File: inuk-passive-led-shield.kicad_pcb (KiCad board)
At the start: 2 copper layers, 100 x 27 mm, 13 parts, among them J1 Conn_01x04_Male, J2 Conn_01x10_Male, J3 Conn_01x02_Male, U1 Logo_NM

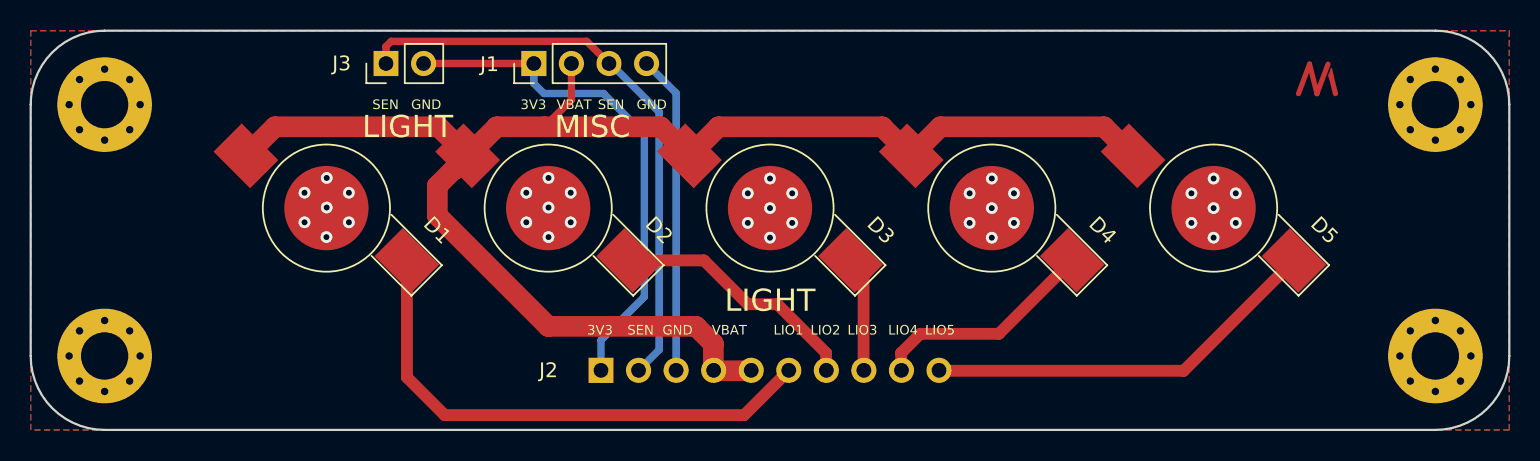
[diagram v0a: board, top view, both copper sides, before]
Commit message: created production files
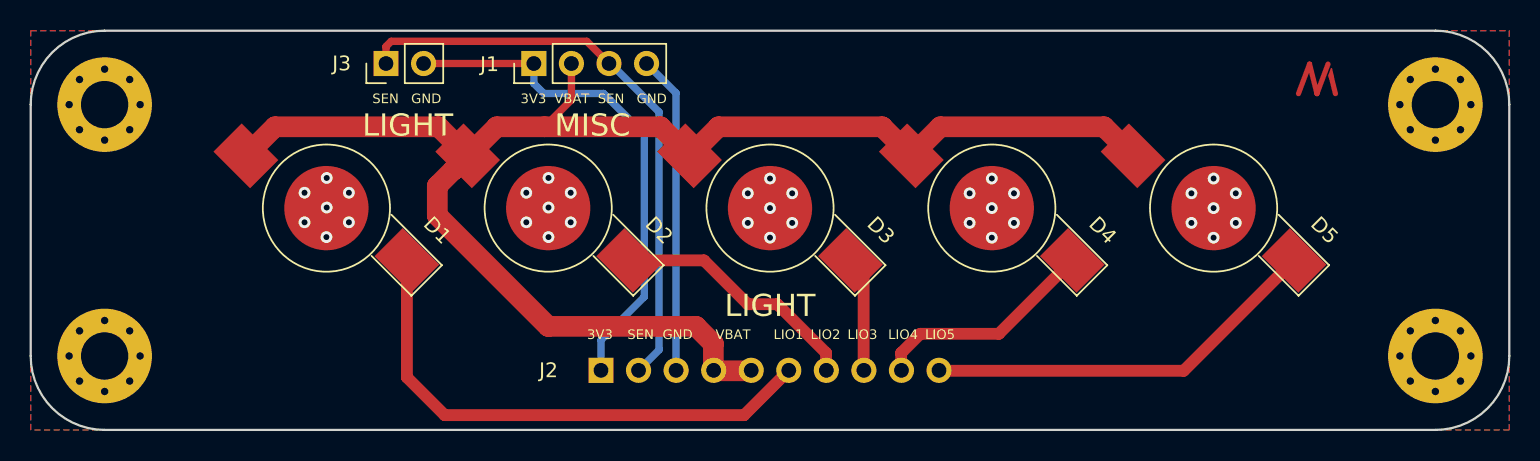
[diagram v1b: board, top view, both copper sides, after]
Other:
- board text added: "Rev: 1.0"
- board text removed: "Rev: 0.9"
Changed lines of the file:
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@@
     (visible_elements FFFFFF7F)
     (pcbplotparams
-      (layerselection 0x00030_ffffffff)
+      (layerselection 0x010ff_ffffffff)
       (usegerberextensions false)
       (usegerberattributes false)
@@
       (drillshape 0)
       (scaleselection 1)
-      (outputdirectory ""))
+      (outputdirectory "production/"))
   )
   (net 0 "")
@@
     )
   )
-  (gr_text LIGHT (at 80.5 124.5) (layer F.SilkS)
+  (gr_text LIGHT (at 80.5 124.4) (layer F.SilkS)
     (effects (font (size 1.5 1.5) (thickness 0.2)))
   )
-  (gr_text MISC (at 93 124.5) (layer F.SilkS)
+  (gr_text MISC (at 93 124.4) (layer F.SilkS)
     (effects (font (size 1.5 1.5) (thickness 0.2)))
   )
-  (gr_text LIGHT (at 105 136.25) (layer F.SilkS)
+  (gr_text LIGHT (at 105 136.6) (layer F.SilkS)
     (effects (font (size 1.5 1.5) (thickness 0.2)))
   )
-  (gr_text SEN (at 79 123) (layer F.SilkS)
-    (effects (font (size 0.65 0.65) (thickness 0.15)))
-  )
-  (gr_text GND (at 81.75 123) (layer F.SilkS)
-    (effects (font (size 0.65 0.65) (thickness 0.15)))
-  )
-  (gr_text GND (at 97 123) (layer F.SilkS)
-    (effects (font (size 0.65 0.65) (thickness 0.15)))
-  )
-  (gr_text SEN (at 94.25 123) (layer F.SilkS)
-    (effects (font (size 0.65 0.65) (thickness 0.15)))
-  )
-  (gr_text VBAT (at 91.75 123) (layer F.SilkS)
-    (effects (font (size 0.65 0.65) (thickness 0.15)))
-  )
-  (gr_text 3V3 (at 89 123) (layer F.SilkS)
-    (effects (font (size 0.65 0.65) (thickness 0.15)))
-  )
-  (gr_text LIO5 (at 116.5 138.25) (layer F.SilkS)
-    (effects (font (size 0.65 0.65) (thickness 0.15)))
-  )
-  (gr_text LIO4 (at 114 138.25) (layer F.SilkS)
-    (effects (font (size 0.65 0.65) (thickness 0.15)))
-  )
-  (gr_text LIO3 (at 111.25 138.25) (layer F.SilkS)
-    (effects (font (size 0.65 0.65) (thickness 0.15)))
-  )
-  (gr_text LIO2 (at 108.75 138.25) (layer F.SilkS)
-    (effects (font (size 0.65 0.65) (thickness 0.15)))
-  )
-  (gr_text LIO1 (at 106.25 138.25) (layer F.SilkS)
-    (effects (font (size 0.65 0.65) (thickness 0.15)))
-  )
-  (gr_text VBAT (at 102.25 138.25) (layer F.SilkS)
-    (effects (font (size 0.65 0.65) (thickness 0.15)))
-  )
-  (gr_text GND (at 98.75 138.25) (layer F.SilkS)
-    (effects (font (size 0.65 0.65) (thickness 0.15)))
-  )
-  (gr_text SEN (at 96.25 138.25) (layer F.SilkS)
-    (effects (font (size 0.65 0.65) (thickness 0.15)))
-  )
-  (gr_text "Rev: 0.9" (at 123.75 121.85) (layer F.Mask)
+  (gr_text SEN (at 79 122.6) (layer F.SilkS)
+    (effects (font (size 0.65 0.65) (thickness 0.15)))
+  )
+  (gr_text GND (at 81.75 122.6) (layer F.SilkS)
+    (effects (font (size 0.65 0.65) (thickness 0.15)))
+  )
+  (gr_text GND (at 97 122.6) (layer F.SilkS)
+    (effects (font (size 0.65 0.65) (thickness 0.15)))
+  )
+  (gr_text SEN (at 94.25 122.6) (layer F.SilkS)
+    (effects (font (size 0.65 0.65) (thickness 0.15)))
+  )
+  (gr_text VBAT (at 91.6 122.6) (layer F.SilkS)
+    (effects (font (size 0.65 0.65) (thickness 0.15)))
+  )
+  (gr_text 3V3 (at 89 122.6) (layer F.SilkS)
+    (effects (font (size 0.65 0.65) (thickness 0.15)))
+  )
+  (gr_text LIO5 (at 116.5 138.55) (layer F.SilkS)
+    (effects (font (size 0.65 0.65) (thickness 0.15)))
+  )
+  (gr_text LIO4 (at 114 138.55) (layer F.SilkS)
+    (effects (font (size 0.65 0.65) (thickness 0.15)))
+  )
+  (gr_text LIO3 (at 111.25 138.55) (layer F.SilkS)
+    (effects (font (size 0.65 0.65) (thickness 0.15)))
+  )
+  (gr_text LIO2 (at 108.75 138.55) (layer F.SilkS)
+    (effects (font (size 0.65 0.65) (thickness 0.15)))
+  )
+  (gr_text LIO1 (at 106.25 138.55) (layer F.SilkS)
+    (effects (font (size 0.65 0.65) (thickness 0.15)))
+  )
+  (gr_text VBAT (at 102.5 138.55) (layer F.SilkS)
+    (effects (font (size 0.65 0.65) (thickness 0.15)))
+  )
+  (gr_text GND (at 98.75 138.55) (layer F.SilkS)
+    (effects (font (size 0.65 0.65) (thickness 0.15)))
+  )
+  (gr_text SEN (at 96.25 138.55) (layer F.SilkS)
+    (effects (font (size 0.65 0.65) (thickness 0.15)))
+  )
+  (gr_text "Rev: 1.0" (at 123.75 121.85) (layer F.Mask)
     (effects (font (size 1 1) (thickness 0.15)))
   )
@@
   (gr_poly (pts (xy 95.5 134.5) (xy 55 134.5) (xy 55 125.5) (xy 95.5 125.5)) (layer B.Mask) (width 0.1))
   (gr_poly (pts (xy 155 134.5) (xy 99.75 134.5) (xy 99.75 125.5) (xy 155 125.5)) (layer B.Mask) (width 0.1))
-  (gr_text 3V3 (at 93.5 138.25) (layer F.SilkS)
-    (effects (font (size 0.65 0.65) (thickness 0.15)))
-  )
+  (gr_text 3V3 (at 93.5 138.55) (layer F.SilkS)
+    (effects (font (size 0.65 0.65) (thickness 0.15)))
+  )
